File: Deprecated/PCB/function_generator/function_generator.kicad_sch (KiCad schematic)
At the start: 30 parts, among them J1 Barrel_Jack, J2 Buttons, J3 LCD, J4 Selector, J5 AD9833, J6 50-ohm BNC, J7 Barrel_Jack, Q1 TIP41, Q2 TIP42, SW1 SW_SPDT, U1 LM358, U2 STM32 Blue Pill, U3 L7805, U4 LM6171, U5 TL071

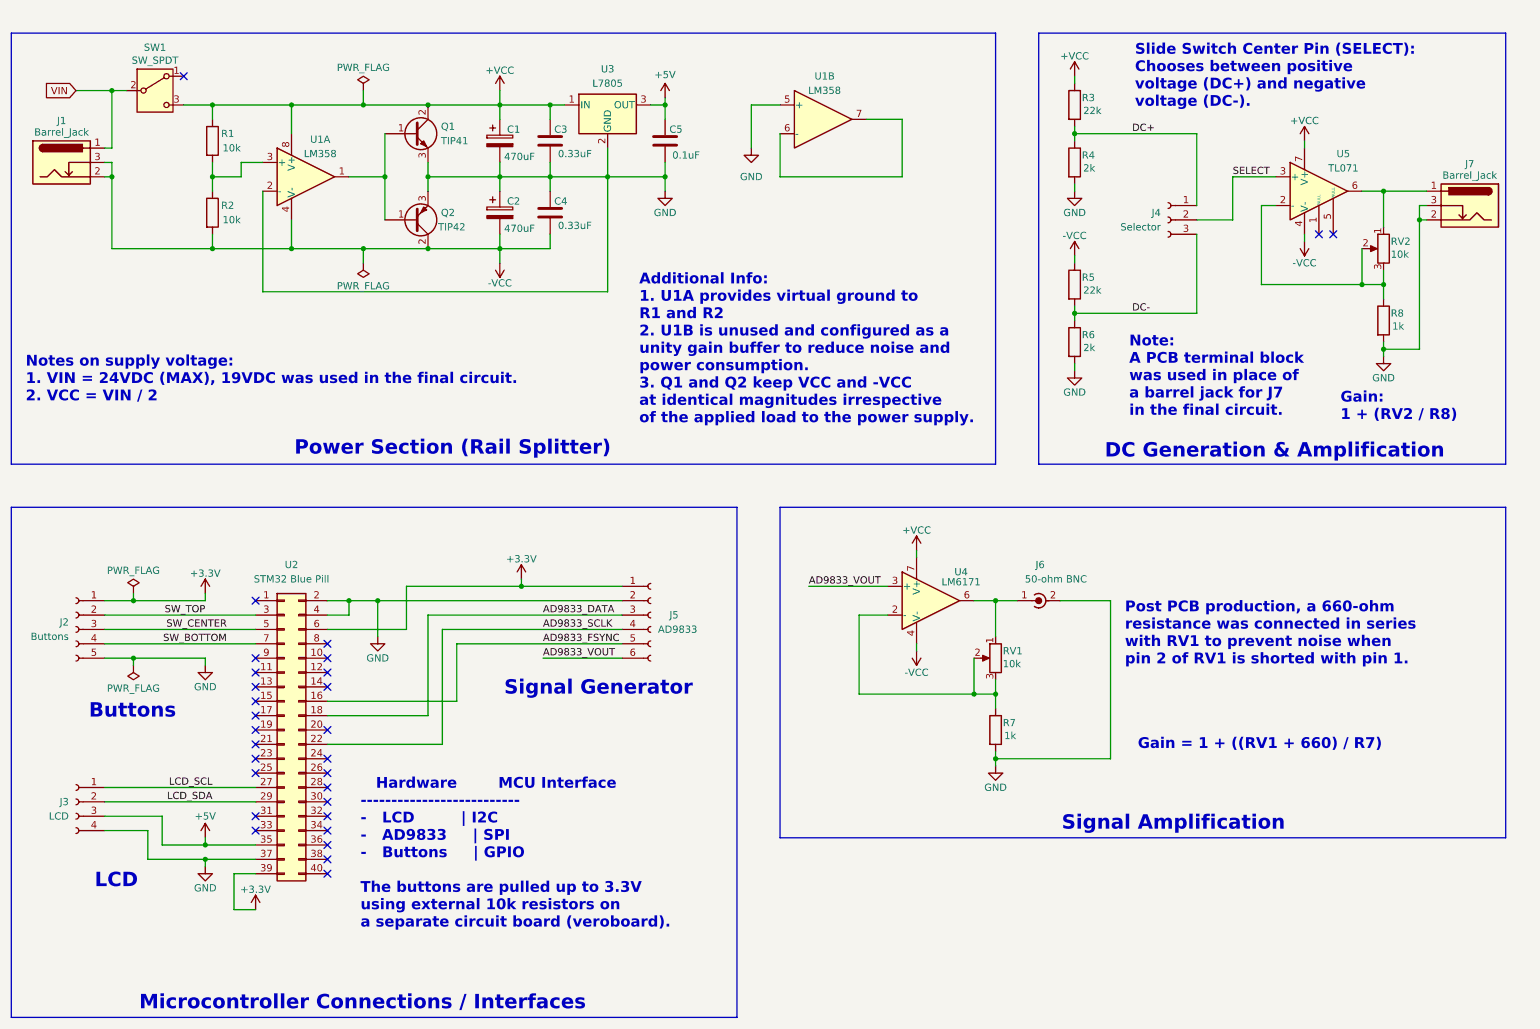
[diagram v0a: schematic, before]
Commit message: Update
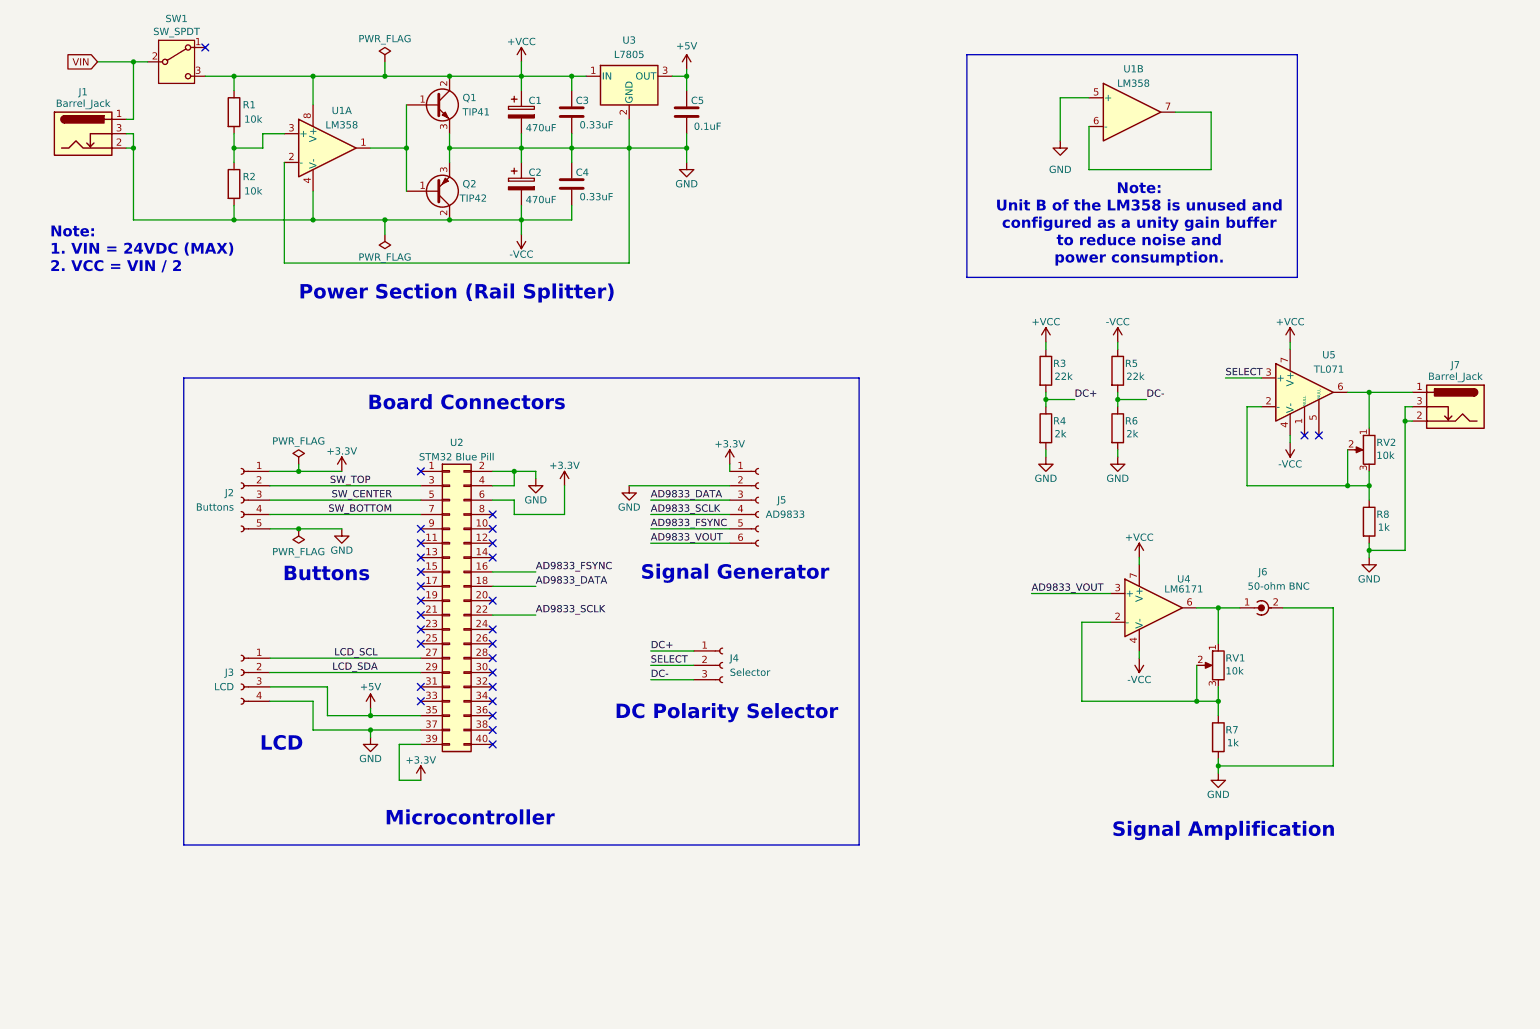
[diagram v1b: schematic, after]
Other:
- note added: "Board Connectors"
- note added: "DC Polarity Selector"
- note added: "Microcontroller"
- note added: "Note: 1. VIN = 24VDC (MAX) 2. VCC = VIN / 2"
- note added: "Note: Unit B of the LM358 is unused and configured as a unity gain buffer to reduce noise and power consumption."
- note removed: "Additional Info: 1. U1A provides virtual ground to R1 and R2 2. U1B is unused and configured as a unity gain buffer to reduce noise and power consumption. 3. Q1 and Q2 keep VCC and -VCC at identical magnitudes irrespective of the applied load to the power supply."
- note removed: "DC Generation & Amplification"
- note removed: "Gain = 1 + ((RV1 + 660) / R7)"
- note removed: "Gain: 1 + (RV2 / R8)"
- note removed: "Hardware MCU Interface -------------------------- - LCD | I2C - AD9833 | SPI - Buttons | GPIO The buttons are pulled up to 3.3V using external 10k resistors on a separate circuit board (veroboard)."
- note removed: "Microcontroller Connections / Interfaces"
- note removed: "Note: A PCB terminal block was used in place of a barrel jack for J7 in the final circuit."
- note removed: "Notes on supply voltage: 1. VIN = 24VDC (MAX), 19VDC was used in the final circuit. 2. VCC = VIN / 2"
- note removed: "Post PCB production, a 660-ohm resistance was connected in series with RV1 to prevent noise when pin 2 of RV1 is shorted with pin 1."
- note removed: "Slide Switch Center Pin (SELECT): Chooses between positive voltage (DC+) and negative voltage (DC-)."
- moved on the sheet: C1, C2, C3, C4, C5, J1, J2, J3, J4, J5, J6, J7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
